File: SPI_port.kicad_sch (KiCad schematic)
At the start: 6 parts, among them J12 Conn_01x06_Female, J27 RJ12_Shielded

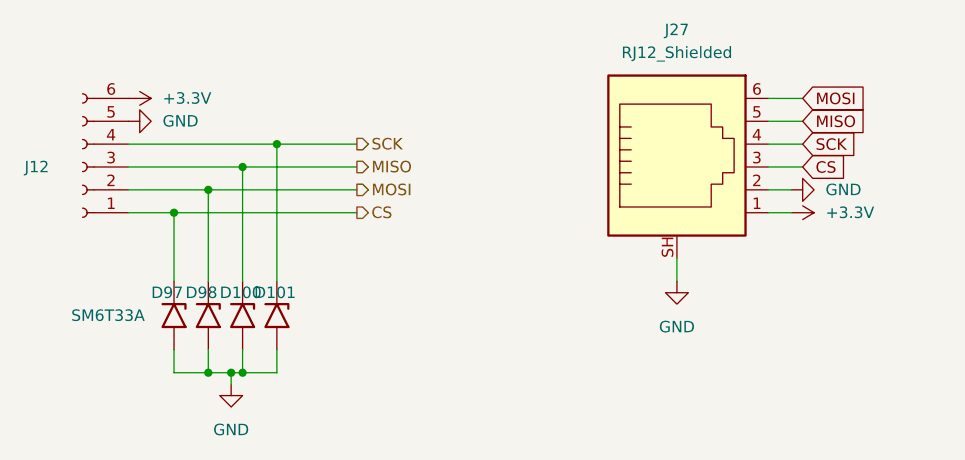
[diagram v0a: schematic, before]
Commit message: v2.1 finished
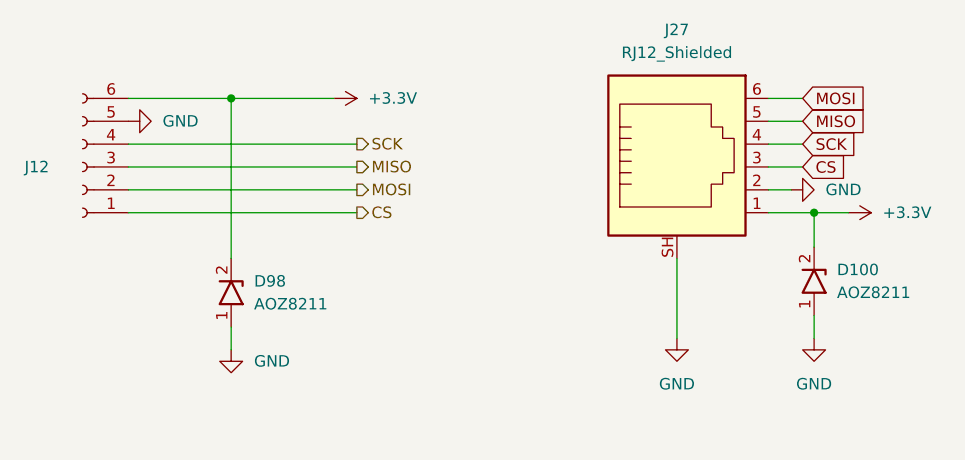
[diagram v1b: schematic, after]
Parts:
- removed D100, D101, D97, D98: SM6T33A, _Diodes:SM2T3V3A, symbol Diode:SM6T33A
- added D100, D98: AOZ8211, _Diodes:AOZ8211, symbol _Diodes:AOZ8211
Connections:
- net +3V3: now also D100.2, D98.2
- net GND: now also D100.1, D98.1
